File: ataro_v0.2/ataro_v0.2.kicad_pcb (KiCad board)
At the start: 4 copper layers, 202.6 x 151 mm, 85 parts, among them J1 4PIN, SW1 ESC, SW10 W, SW11 E, SW12 R, SW13 T, SW14 Y, SW15 CAPSLOCK, SW16 A, SW17 S, SW18 D, SW19 F, SW2 TILDE, SW20 G, SW21 {, SW22 SHIFT, SW23 Z, SW24 X, SW25 C, SW26 V, SW27 B, SW28 }, SW29 CTRL, SW3 1, SW30 ^, SW31 v, SW32 SUPER, SW33 ALT, SW34 SPACE, SW35 BACKSPACE, SW4 2, SW5 3, SW6 4, SW7 5, SW8 TAB, SW9 Q, U1 ProMicro

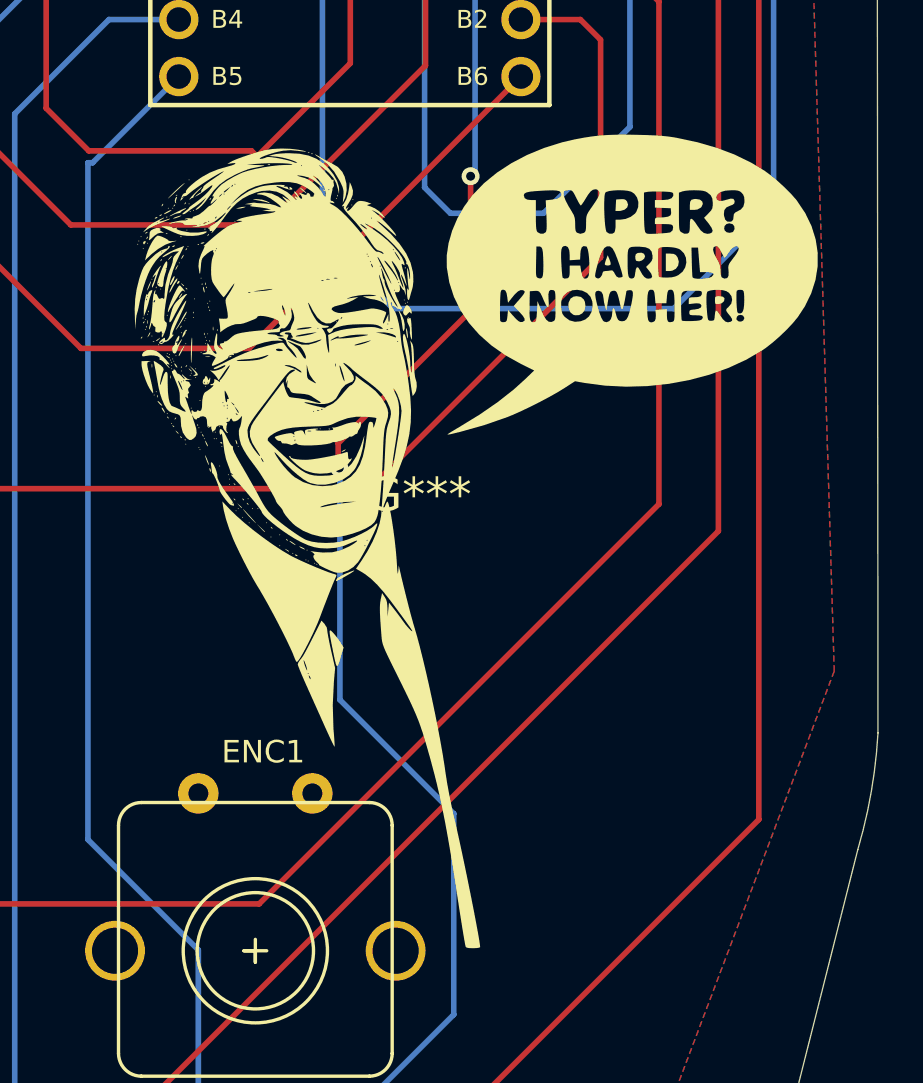
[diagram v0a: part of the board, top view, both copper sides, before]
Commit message: Final iteration of v0.2 for JLCPCB prod
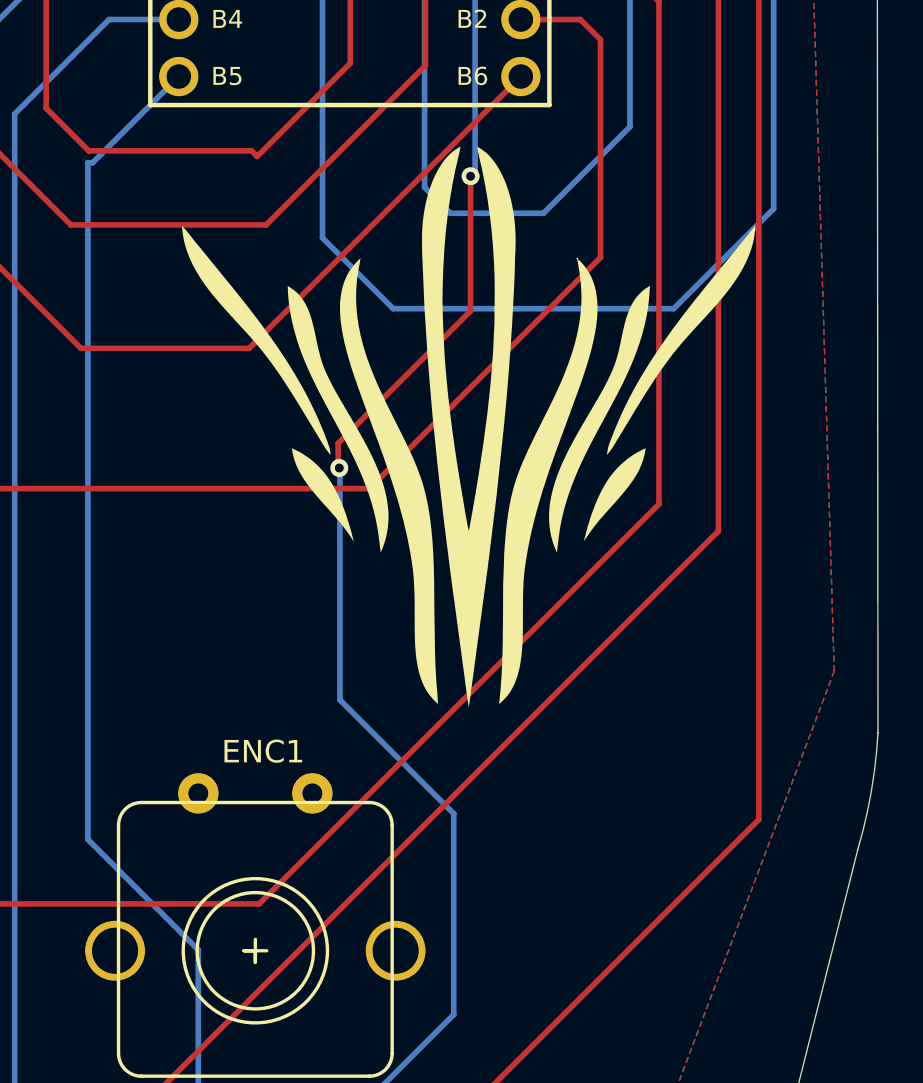
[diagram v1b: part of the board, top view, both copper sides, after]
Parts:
- removed G*** (x2): LOGO, LOGO
